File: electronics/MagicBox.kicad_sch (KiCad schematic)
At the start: 16 parts, among them SW1_1 SW_Push, SW1_2 SW_Push, SW1_3 SW_Push, SW1_4 SW_Push, SW5 SW_DPST_x2, SW5 SW_Push, SW7 RotaryEncoder_Switch, U1.U1 ESP32-WROOM-32, U1.U2 L7805

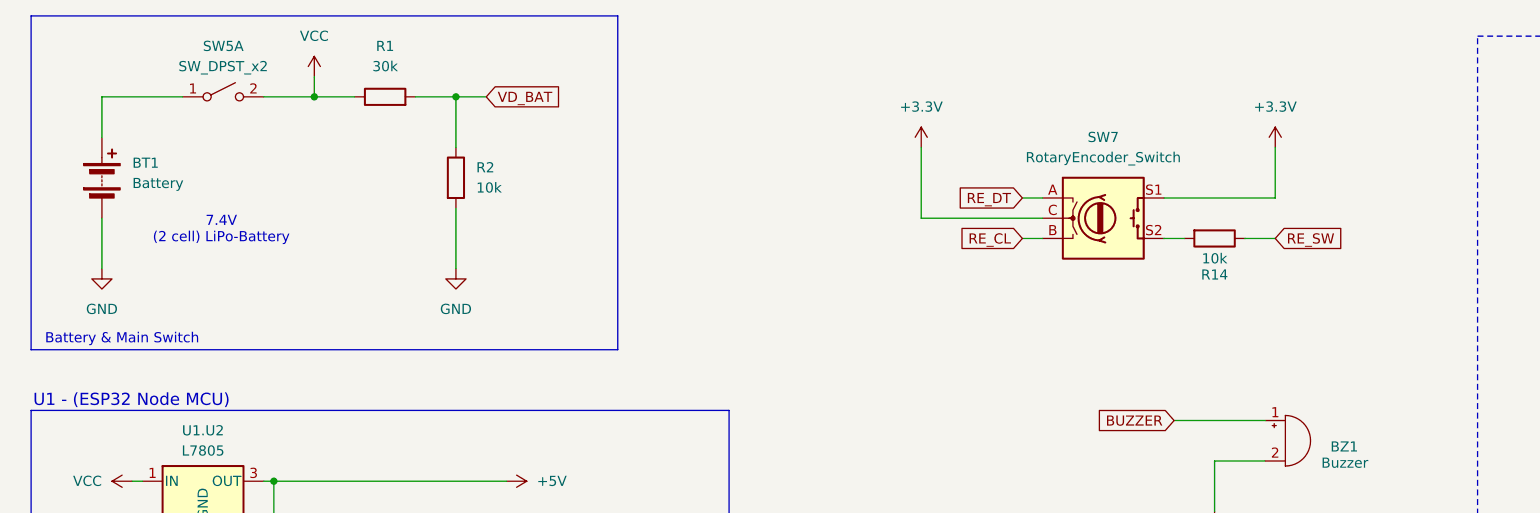
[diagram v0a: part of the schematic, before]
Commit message: small electronics and priting additions
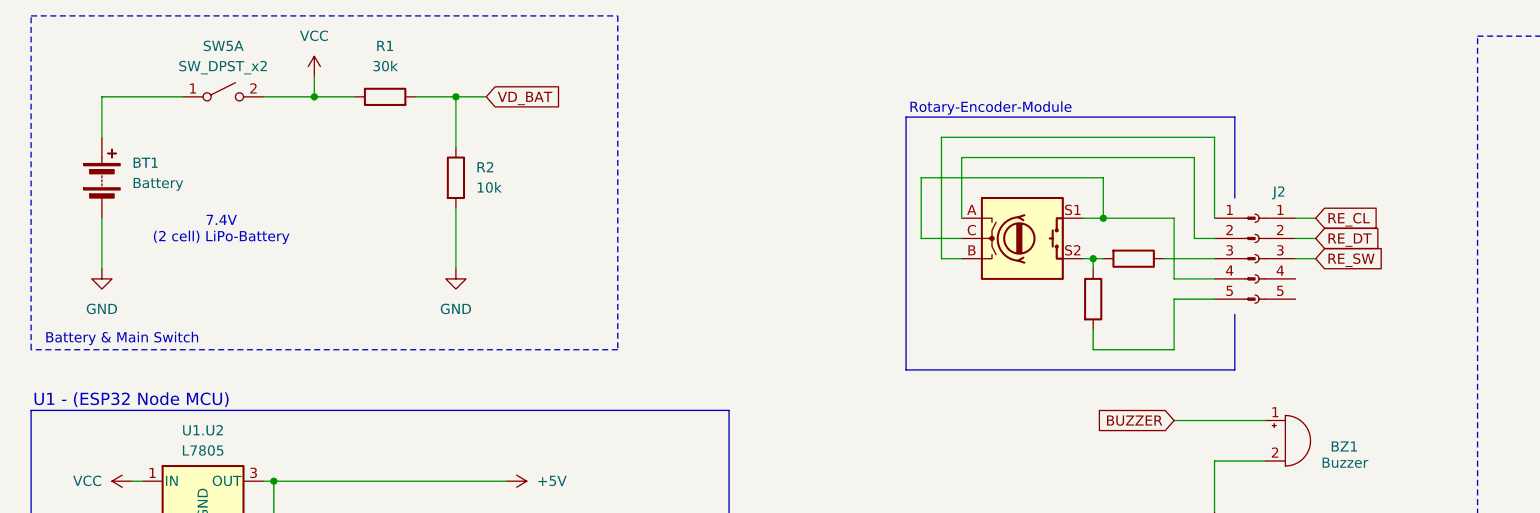
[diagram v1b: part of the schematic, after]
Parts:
- added J1: Conn_01x05_Pin, symbol Connector:Conn_01x05_Pin
- added J2: Conn_01x05_Socket, symbol Connector:Conn_01x05_Socket
- added R3: 10k, symbol Device:R
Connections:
- net +3.3V: no longer SW7.C, SW7.S1
- net RE_CL: now also J2.1 (Pin_1); no longer SW7.B
- net RE_DT: now also J2.2 (Pin_2); no longer SW7.A
- net RE_SW: now also J2.3 (Pin_3); no longer R14.1
- net at R14.2, SW7.S2: now also R3.1
- new net: J1.5 (Pin_5), R3.2
- new net: J1.3 (Pin_3), R14.1
- new net: J1.1 (Pin_1), SW7.B
- new net: J1.2 (Pin_2), SW7.A
- new net: J1.4 (Pin_4), SW7.C, SW7.S1
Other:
- note added: "Rotary-Encoder-Module"
